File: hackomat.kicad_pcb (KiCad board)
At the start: 2 copper layers, 95 x 90 mm, 54 parts, among them IC1 MOC3021M, IC10 MOC3021M, IC11 MOC3021M, IC12 MOC3021M, IC13 MOC3021M, IC14 MOC3021M, IC15 MOC3021M, IC16 MOC3021M, IC17 MOC3021M, IC18 MOC3021M, IC19 MOC3021M, IC2 MOC3021M, IC20 MOC3021M, IC21 MOC3021M, IC22 MOC3021M, IC23 MOC3021M, IC24 MOC3021M, IC25 MOC3021M, IC26 MOC3021M, IC27 MOC3021M, IC28 MOC3021M, IC29 MOC3021M, IC3 MOC3021M, IC30 MOC3021M, IC31 MOC3021M, IC32 MOC3021M, IC33 MOC3021M, IC34 MOC3021M, IC35 MOC3021M, IC36 MOC3021M, IC37 MOC3021M, IC38 MOC3021M, IC39 MOC3021M, IC4 MOC3021M, IC40 MOC3021M, IC41 MOC3021M, IC42 MOC3021M, IC5 MOC3021M, IC6 MOC3021M, IC7 MOC3021M, IC8 MOC3021M, IC9 MOC3021M, J1 RJ45, P1 CONN_02X22, P2 CONN_02X08, P35 CONN_01X01, P36 CONN_01X01, P42 CONN_01X01

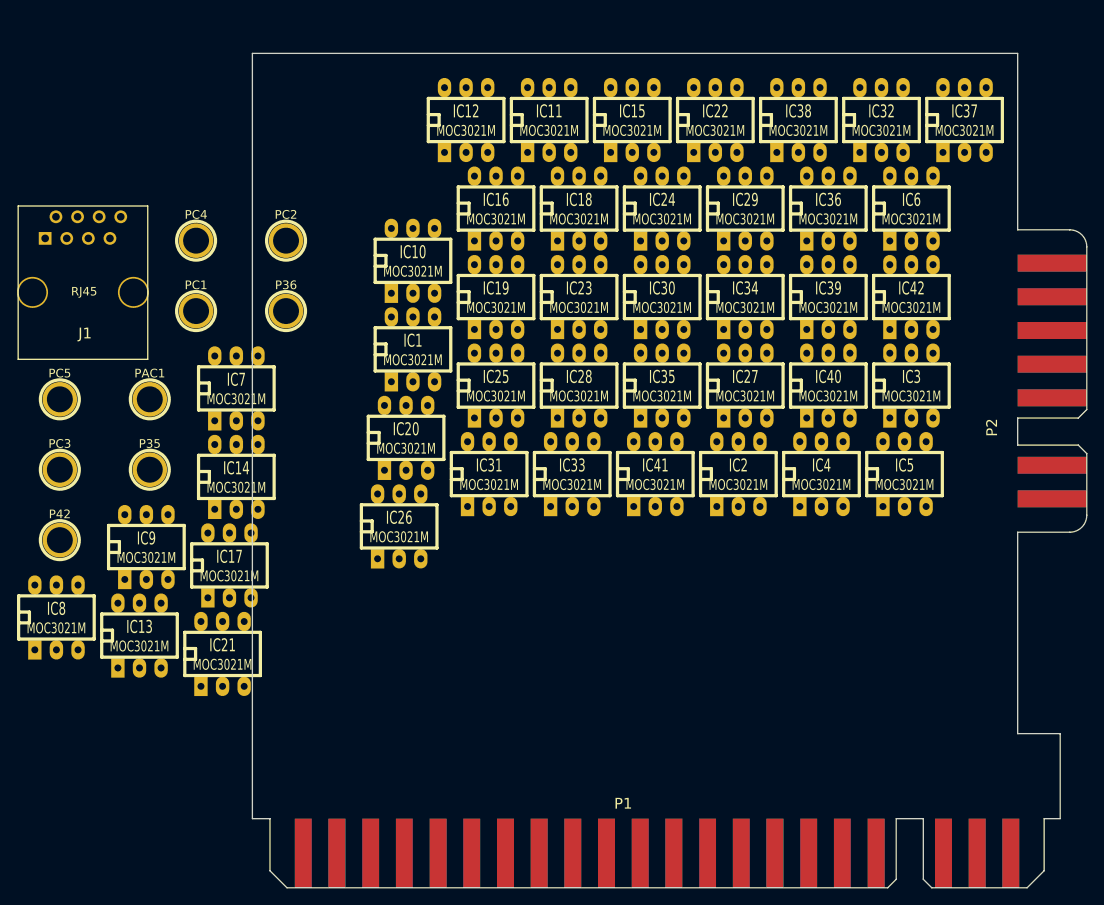
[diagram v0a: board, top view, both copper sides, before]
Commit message: place all triacs and other parts on board in order
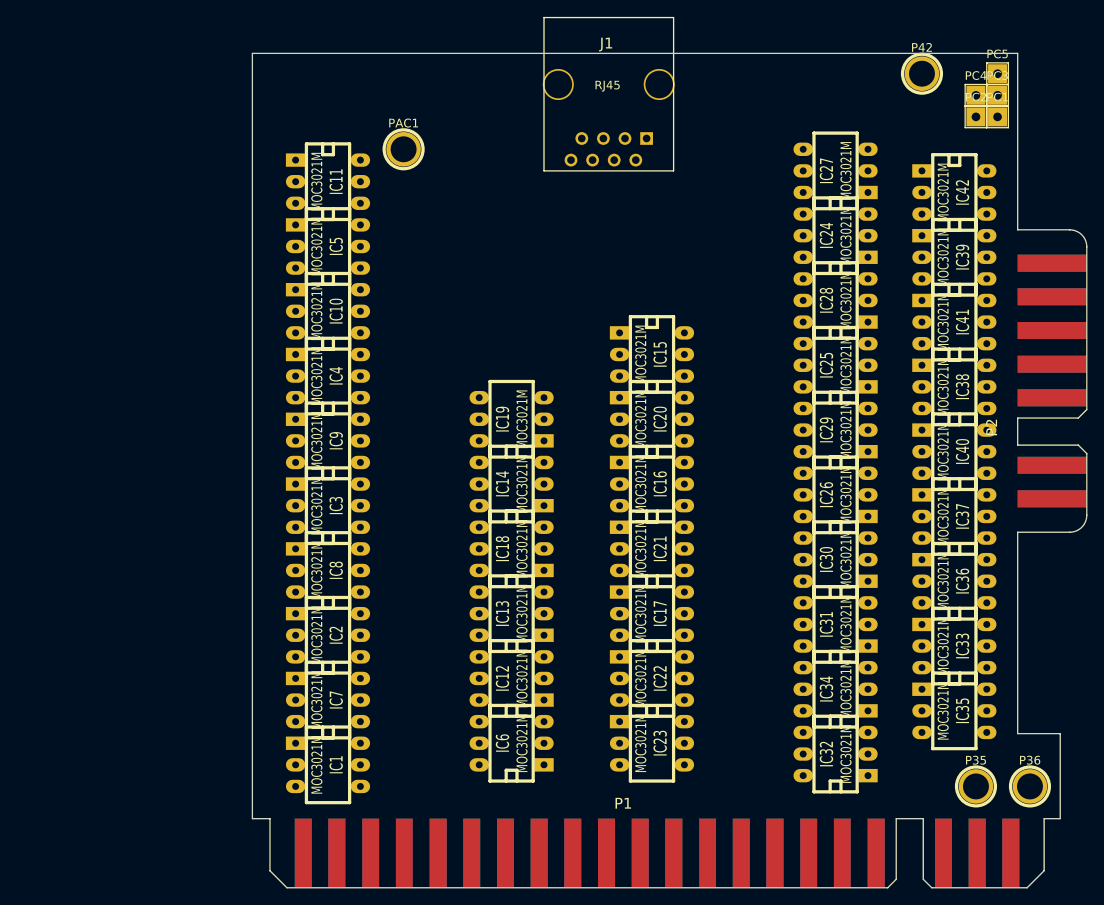
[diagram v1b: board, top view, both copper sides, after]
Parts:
- PC1, PC2, PC3, PC4, PC5: footprint Connect:1pin -> Pin_Headers:Pin_Header_Straight_1x01
- moved PC3 118.7 mm to (247.7, 74.9)
- moved PC5 116.7 mm to (247.7, 72.4)
- moved P42 115.3 mm to (238.8, 72.4)
- moved P35 104.1 mm to (245.1, 156.2)
- moved P36 103.8 mm to (251.5, 156.2)
- moved PC1 97.0 mm to (247.7, 77.5)
- moved PC4 93.3 mm to (245.1, 74.9)
- moved PC2 82.4 mm to (245.1, 77.5)
- moved IC6 78.5 mm to (190.5, 151.1), turned to 90 degrees
- moved IC32 74.8 mm to (228.6, 152.4), turned to 90 degrees
- moved IC5 72.9 mm to (168.9, 92.7), turned to 270 degrees
- moved IC3 70.0 mm to (168.9, 123.2), turned to 270 degrees
- moved J1 66.5 mm to (201.9, 73.7), turned to 180 degrees
- moved IC22 66.1 mm to (207.0, 143.5), turned to 270 degrees
- moved IC12 65.9 mm to (190.5, 143.5), turned to 90 degrees
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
